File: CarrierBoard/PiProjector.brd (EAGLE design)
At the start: 86.4 x 54.6 mm, 79 parts, among them P8 PINHEAD2X23, P9 PINHEAD2X23, Q2 BSS84, X1 24MHz, X2 12Mhz

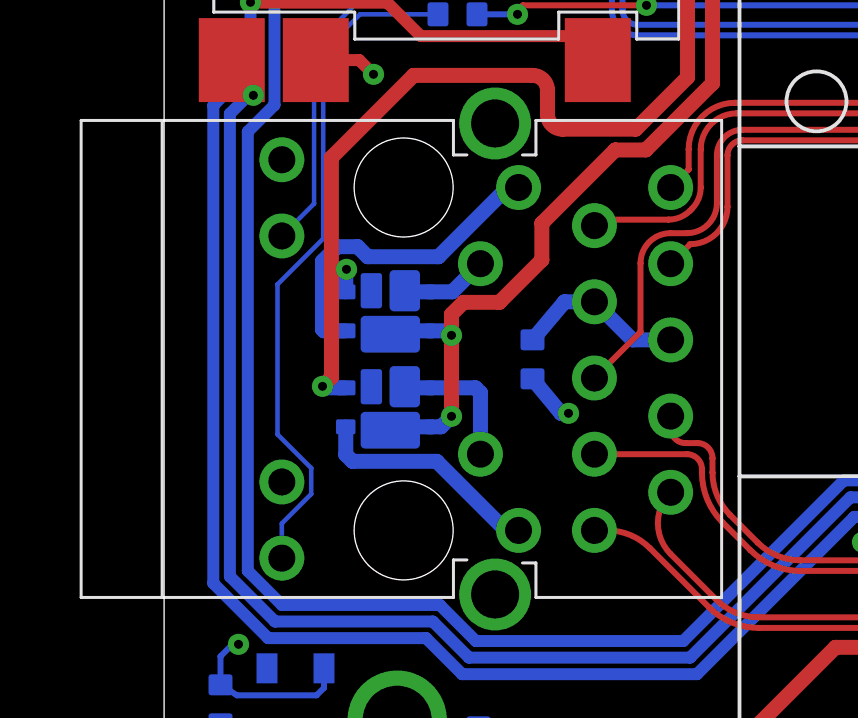
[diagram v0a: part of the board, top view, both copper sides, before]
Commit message: Modified POE route  to avoid clearence issues
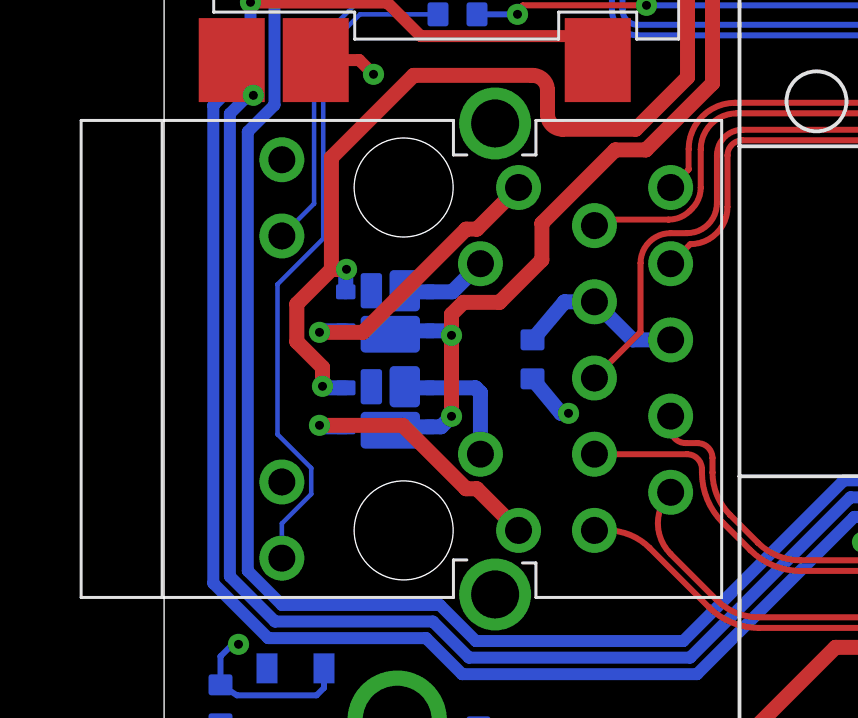
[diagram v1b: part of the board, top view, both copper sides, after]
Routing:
- net N$43: track 10.9 -> 9.53 mm, vias 0 -> 1
- net N$33: track 7.73 -> 8.98 mm, vias 0 -> 1
- net POE-: track 41.9 -> 42.6 mm
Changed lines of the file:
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@@
 <layer number="13" name="Route13" color="21" fill="1" visible="no" active="no"/>
 <layer number="14" name="Route14" color="22" fill="1" visible="no" active="no"/>
-<layer number="15" name="Route15" color="23" fill="1" visible="yes" active="yes"/>
+<layer number="15" name="Route15" color="23" fill="1" visible="no" active="yes"/>
 <layer number="16" name="Bottom" color="1" fill="1" visible="yes" active="yes"/>
 <layer number="17" name="Pads" color="2" fill="1" visible="yes" active="yes"/>
@@
 <wire x1="-37.125" y1="5.375" x2="-37.1" y2="5.4" width="0.5" layer="16"/>
 <contactref element="P8" pad="6"/>
-<wire x1="-37.6" y1="5.4" x2="-37.1" y2="5.4" width="0.5" layer="1"/>
-<wire x1="-37.9" y1="1.5" x2="-37.6" y2="1.8" width="0.5" layer="1"/>
-<wire x1="-37.6" y1="5.4" x2="-37.6" y2="1.8" width="0.5" layer="1"/>
+<wire x1="-37.1" y1="5.4" x2="-37.6" y2="5.4" width="0.5" layer="1"/>
 <wire x1="-34.86303125" y1="11.8654" x2="-37.603" y2="9.12543125" width="0.5" layer="1"/>
 <wire x1="-37.603" y1="9.12543125" x2="-37.603" y2="5.4" width="0.5" layer="1"/>
@@
 <wire x1="-30.4" y1="11.3654" x2="-30.9" y2="11.8654" width="0.5" layer="1" curve="90"/>
 <wire x1="-30.9" y1="11.8654" x2="-34.86303125" y2="11.8654" width="0.5" layer="1"/>
+<wire x1="-37.9" y1="2.13141875" x2="-37.9" y2="1.5" width="0.5" layer="1"/>
+<wire x1="-38.7556" y1="2.98701875" x2="-37.9" y2="2.13141875" width="0.5" layer="1"/>
+<wire x1="-37.6" y1="5.4" x2="-38.7556" y2="4.2444" width="0.5" layer="1"/>
+<wire x1="-38.7556" y1="4.2444" x2="-38.7556" y2="2.98701875" width="0.5" layer="1"/>
 </signal>
 <signal name="N$37">
@@
 <contactref element="D1" pad="3"/>
 <contactref element="U$5" pad="11"/>
-<wire x1="-31.72474375" y1="8.128" x2="-31.365" y2="8.128" width="0.5" layer="16"/>
-<wire x1="-37.85" y1="3.35" x2="-37.125" y2="3.35" width="0.5" layer="16"/>
-<wire x1="-37.85" y1="3.35" x2="-37.9" y2="3.4" width="0.5" layer="16"/>
-<wire x1="-37.9" y1="5.66858125" x2="-37.41298125" y2="6.1556" width="0.5" layer="16"/>
-<wire x1="-37.41298125" y1="6.1556" x2="-36.72803125" y2="6.1556" width="0.5" layer="16"/>
-<wire x1="-36.72803125" y1="6.1556" x2="-36.39243125" y2="5.82" width="0.5" layer="16"/>
-<wire x1="-37.9" y1="3.4" x2="-37.9" y2="5.66858125" width="0.5" layer="16"/>
-<wire x1="-36.39243125" y1="5.82" x2="-34.03274375" y2="5.82" width="0.5" layer="16"/>
-<wire x1="-34.03274375" y1="5.82" x2="-31.72474375" y2="8.128" width="0.5" layer="16"/>
+<via x="-38" y="3.3" extent="1-16" drill="0.3"/>
+<wire x1="-31.365" y1="8.128" x2="-32.7526" y2="6.7404" width="0.5" layer="1"/>
+<wire x1="-32.7526" y1="6.7404" x2="-33.11234375" y2="6.7404" width="0.5" layer="1"/>
+<wire x1="-36.55274375" y1="3.3" x2="-38" y2="3.3" width="0.5" layer="1"/>
+<wire x1="-33.11234375" y1="6.7404" x2="-36.55274375" y2="3.3" width="0.5" layer="1"/>
+<wire x1="-38" y1="3.3" x2="-37.95" y2="3.35" width="0.5" layer="16"/>
+<wire x1="-37.95" y1="3.35" x2="-37.125" y2="3.35" width="0.5" layer="16"/>
 </signal>
 <signal name="N$33">
 <contactref element="D2" pad="3"/>
 <contactref element="U$5" pad="14"/>
-<wire x1="-37.125" y1="0.15" x2="-37.125" y2="-0.775" width="0.5" layer="16"/>
-<wire x1="-37.125" y1="-0.775" x2="-36.9" y2="-1" width="0.5" layer="16"/>
-<wire x1="-36.9" y1="-1" x2="-34.09156875" y2="-1" width="0.5" layer="16"/>
-<wire x1="-31.78956875" y1="-3.302" x2="-31.365" y2="-3.302" width="0.5" layer="16"/>
-<wire x1="-34.09156875" y1="-1" x2="-31.78956875" y2="-3.302" width="0.5" layer="16"/>
+<wire x1="-37.125" y1="0.15" x2="-37.95" y2="0.15" width="0.5" layer="16"/>
+<wire x1="-37.95" y1="0.15" x2="-38" y2="0.2" width="0.5" layer="16"/>
+<via x="-38" y="0.2" extent="1-16" drill="0.3"/>
+<wire x1="-33.11234375" y1="-1.9144" x2="-32.7526" y2="-1.9144" width="0.5" layer="1"/>
+<wire x1="-32.7526" y1="-1.9144" x2="-31.365" y2="-3.302" width="0.5" layer="1"/>
+<wire x1="-38" y1="0.2" x2="-35.22674375" y2="0.2" width="0.5" layer="1"/>
+<wire x1="-35.22674375" y1="0.2" x2="-33.11234375" y2="-1.9144" width="0.5" layer="1"/>
 </signal>
 <signal name="N$34">
